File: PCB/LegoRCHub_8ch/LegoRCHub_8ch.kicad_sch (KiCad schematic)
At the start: 35 parts, among them J1 Conn_01x02, J2 Conn_01x02, J3 Conn_01x02, J4 Conn_01x02, J5 Conn_01x02, J6 Conn_01x03, J7 Conn_01x03, J8 Conn_01x03, J9 Conn_01x02, U1 DRV8872DDA, U2 DRV8872DDA, U3 DRV8872DDA, U4 DRV8872DDA, U5 DRV8872DDA, U6 AMS1117-5.0, U7 ATtiny3226-X

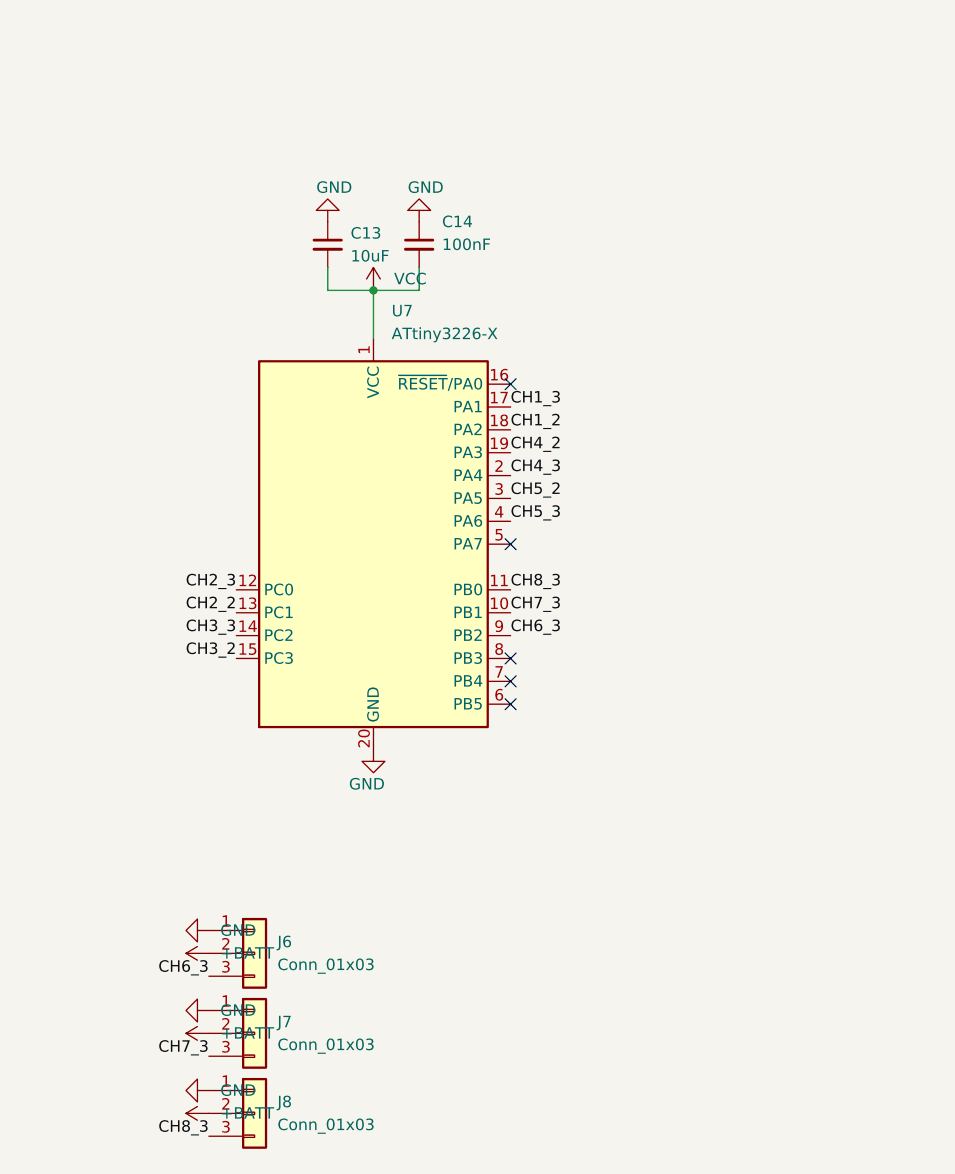
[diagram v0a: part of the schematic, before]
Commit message: LegoRCHub_8ch: finished PCB (beta 1)
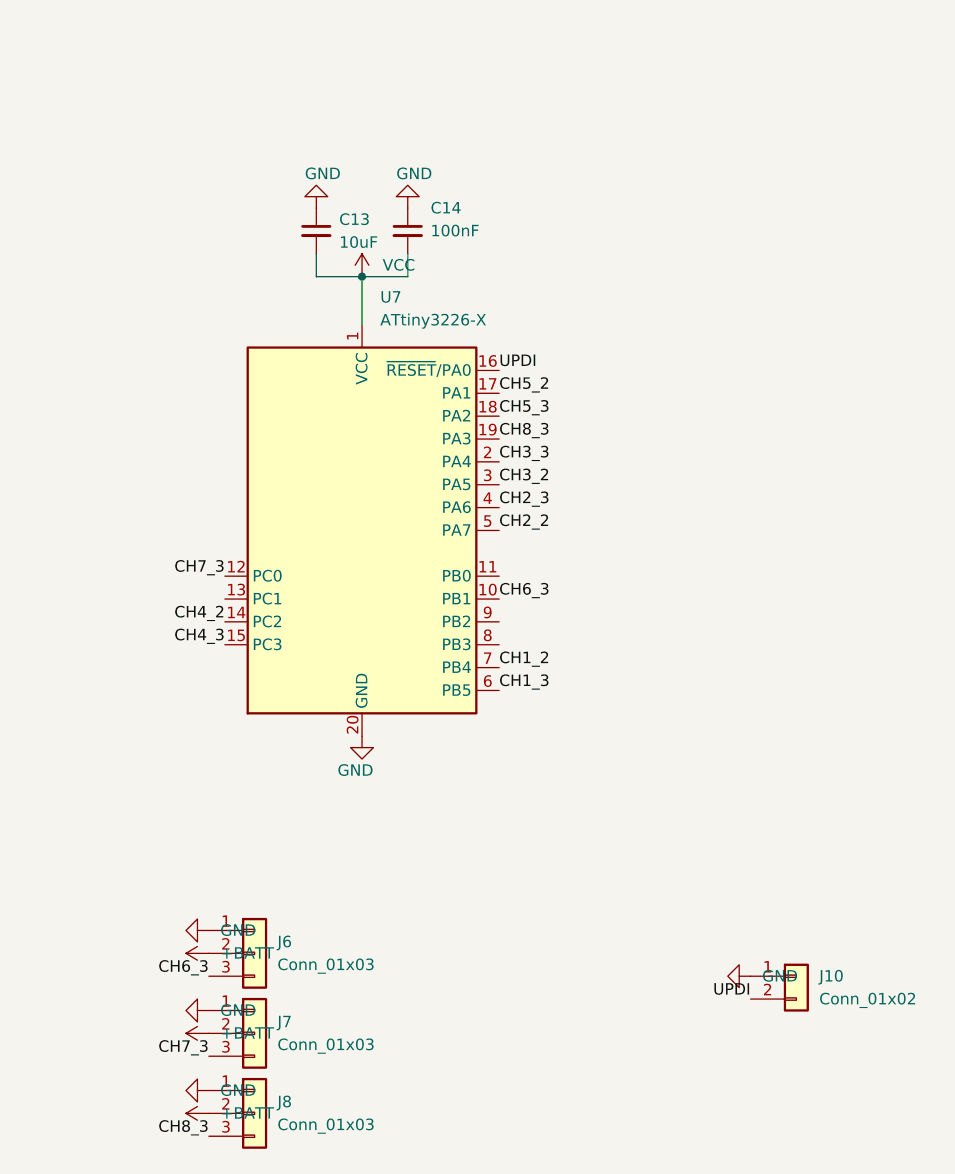
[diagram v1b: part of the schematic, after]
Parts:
- added J10: Conn_01x02, Connector_PinHeader_2.54mm:PinHeader_1x02_P2.54mm_Vertical, symbol Connector_Generic:Conn_01x02
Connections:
- net CH1_2: now also U7.7 (PB4); no longer U7.18 (PA2)
- net CH1_3: now also U7.6 (PB5); no longer U7.17 (PA1)
- net CH2_2: now also U7.5 (PA7); no longer U7.13 (PC1)
- net CH2_3: now also U7.4 (PA6); no longer U7.12 (PC0)
- net CH3_2: now also U7.3 (PA5); no longer U7.15 (PC3)
- net CH3_3: now also U7.2 (PA4); no longer U7.14 (PC2)
- net CH4_2: now also U7.14 (PC2); no longer U7.19 (PA3)
- net CH4_3: now also U7.15 (PC3); no longer U7.2 (PA4)
- net CH5_2: now also U7.17 (PA1); no longer U7.3 (PA5)
- net CH5_3: now also U7.18 (PA2); no longer U7.4 (PA6)
- net CH6_3: now also U7.10 (PB1); no longer U7.9 (PB2)
- net CH7_3: now also U7.12 (PC0); no longer U7.10 (PB1)
- net CH8_3: now also U7.19 (PA3); no longer U7.11 (PB0)
- net GND: now also J10.1 (Pin_1)
- net UPDI: now reaches U7.16 (~{RESET}/PA0)
- net UPDI: now also J10.2 (Pin_2)
- no-connect marks 5 -> 0
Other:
- moved on the sheet: C13, C14, U7
